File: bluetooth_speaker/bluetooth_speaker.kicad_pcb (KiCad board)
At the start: 2 copper layers, 40 parts, among them J1 Conn_Coaxial, J2 USB_C_Receptacle_USB2.0_16P, J3 282836-4, U1 MAX98357A, U2 XL4015, U3 CP2102N-A01-GQFN28, U4 ESP32-D0WD-V3, Y1 40MHz(±10 ppm)

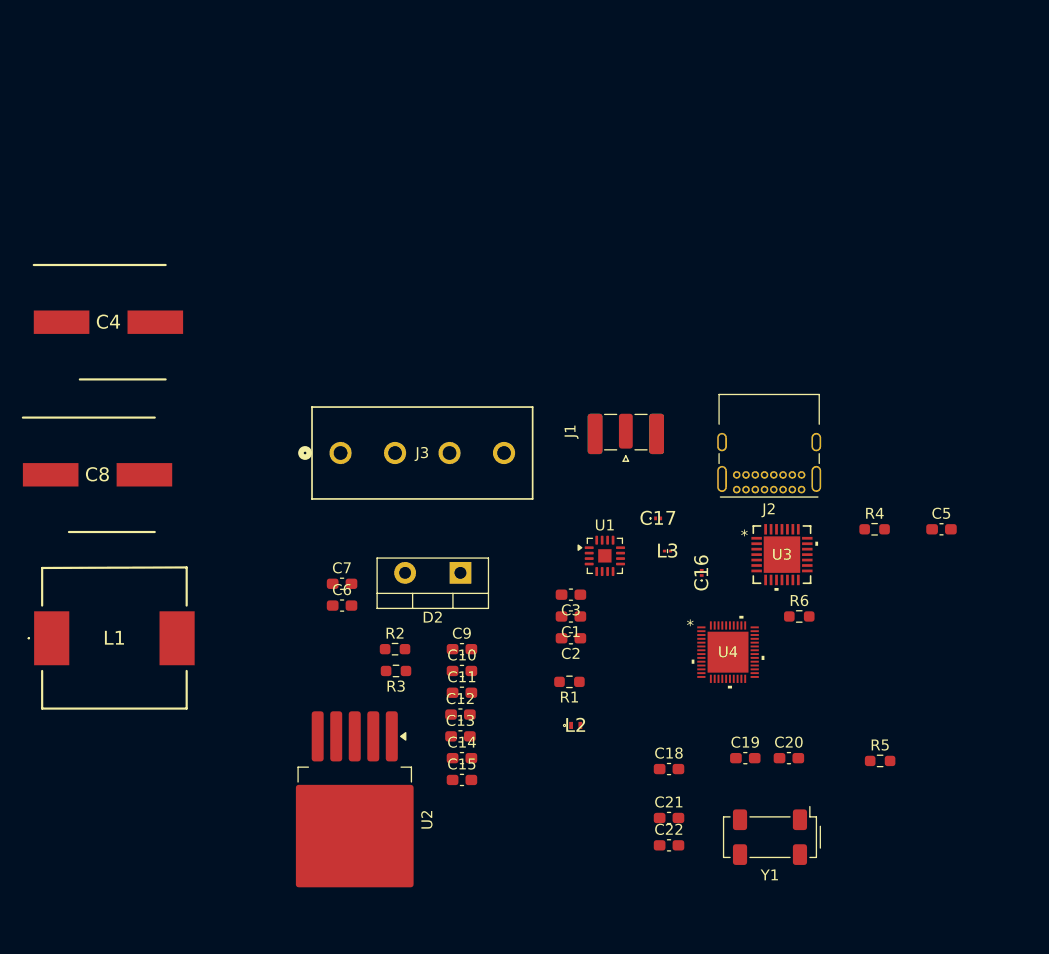
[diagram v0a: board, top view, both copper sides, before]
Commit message: pcb layout
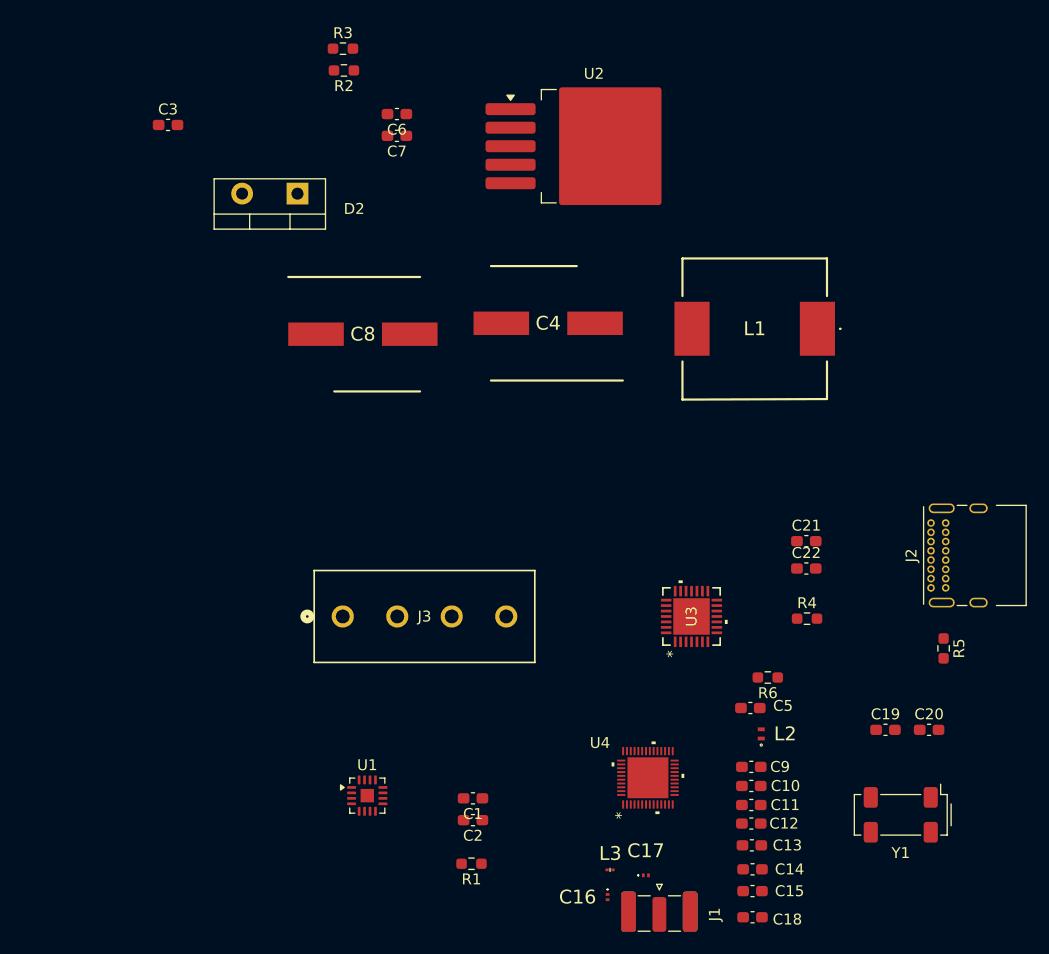
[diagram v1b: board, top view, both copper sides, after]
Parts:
- moved U2 65.6 mm to (119.2, 40.9), turned to 0 degrees
- moved L1 65.3 mm to (134.0, 57.6), turned to 180 degrees
- moved R3 57.3 mm to (96.2, 31.9), turned to 0 degrees
- moved C3 56.8 mm to (80.2, 38.9), turned to 0 degrees
- moved R2 53.3 mm to (96.3, 33.9), turned to 180 degrees
- moved C6 45.4 mm to (101.2, 37.9), turned to 180 degrees
- moved J1 44.4 mm to (125.2, 111.3), turned to -90 degrees
- moved C7 41.4 mm to (101.2, 39.9), turned to 180 degrees
- moved C4 40.3 mm to (115.0, 57.1), turned to 180 degrees
- moved D2 37.9 mm to (92.0, 45.2)
- moved C17 32.8 mm to (124.0, 107.8)
- moved C16 31.0 mm to (120.5, 109.8), turned to -90 degrees
- moved U1 31.0 mm to (98.5, 100.4)
- moved L3 29.7 mm to (120.7, 107.2)
- moved C9 28.7 mm to (133.7, 97.8), turned to 180 degrees
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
